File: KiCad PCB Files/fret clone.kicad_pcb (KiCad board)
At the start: 2 copper layers, 141.1 x 26 mm, 7 parts, among them J1 Conn_01x03_Pin, J2 Conn_01x03_Pin

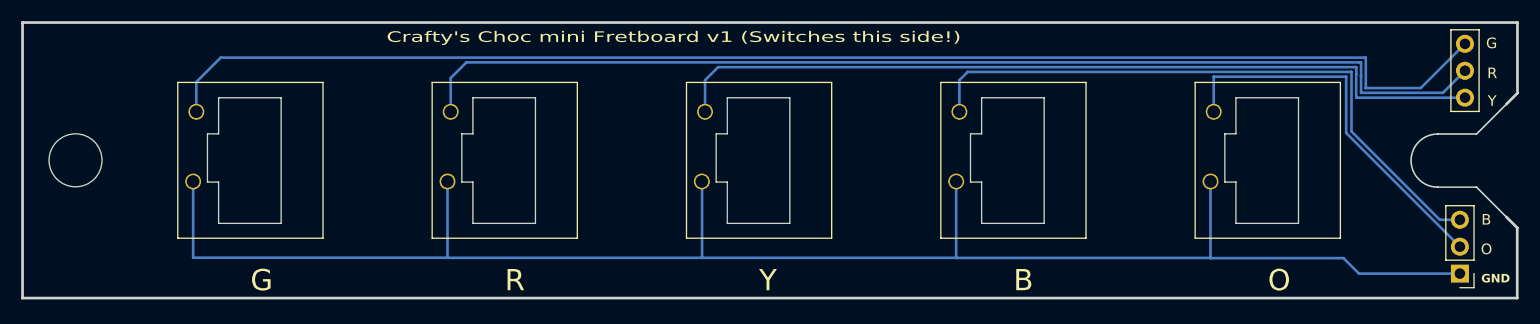
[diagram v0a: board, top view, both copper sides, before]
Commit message: add the things new LED
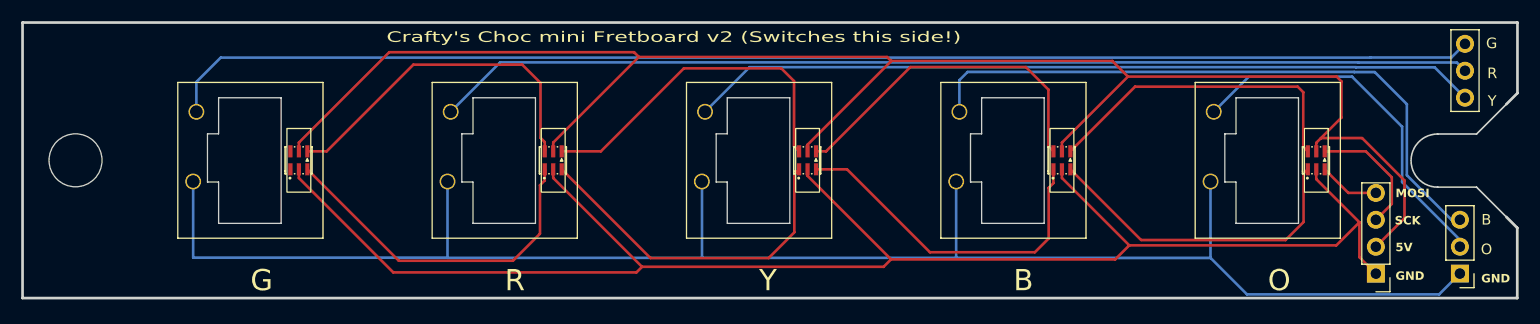
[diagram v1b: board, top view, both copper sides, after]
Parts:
- added J3: Conn_01x04_Pin, Connector_PinHeader_2.54mm:PinHeader_1x04_P2.54mm_Vertical, F.Cu at (127.7, -9.93)
- added LED1: ~, sk9822-ec20:SK9822-EC20, F.Cu at (122.1, -13.0)
- added LED2: ~, sk9822-ec20:SK9822-EC20, F.Cu at (98.1, -13.0)
- added LED3: ~, sk9822-ec20:SK9822-EC20, F.Cu at (74.1, -13.0)
- added LED4: ~, sk9822-ec20:SK9822-EC20, F.Cu at (50.1, -13.0)
- added LED5: ~, sk9822-ec20:SK9822-EC20, F.Cu at (26.1, -13.0)
- CH1, CH2, CH3, CH4, CH5: footprint PCM_Switch_Keyboard_Kailh:SW_Kailh_Choc_Mini_1.00u -> PCM_Switch_Keyboard_Kailh:SW_Kailh_Choc_Mini
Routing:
- net Net-(J3-Pin_3): track 0.00 -> 162.0 mm
- net /GND: track 0.00 -> 153.0 mm
- net Net-(LED4-SDO): track 0.00 -> 32.8 mm
- net Net-(LED4-CKO): track 0.00 -> 32.7 mm
- net Net-(LED3-SDO): track 0.00 -> 32.6 mm
- net Net-(LED3-CKO): track 0.00 -> 32.5 mm
- net Net-(LED2-SDO): track 0.00 -> 32.4 mm
- net Net-(LED2-CKO): track 0.00 -> 32.1 mm
- net Net-(LED1-SDO): track 0.00 -> 30.6 mm
- net Net-(LED1-CKO): track 0.00 -> 30.5 mm
- net Net-(J3-Pin_2): track 0.00 -> 12.0 mm
- net Net-(J3-Pin_1): track 0.00 -> 5.75 mm
- net Net-(J2-Pin_2): track 103.2 -> 98.0 mm
- net Net-(J2-Pin_3): track 128.1 -> 124.0 mm
- net Net-(J2-Pin_1): track 78.1 -> 74.6 mm
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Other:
- board text added: "5V"
- board text added: "Crafty's Choc mini Fretboard v2"
- board text added: "Crafty's Choc mini Fretboard v2 (Switches this side!)"
- board text added: "MOSI"
- board text added: "SCK"
- board text removed: "Crafty's Choc mini Fretboard v1"
- board text removed: "Crafty's Choc mini Fretboard v1 (Switches this side!)"
